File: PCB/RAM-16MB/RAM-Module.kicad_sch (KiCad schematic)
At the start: 0 parts

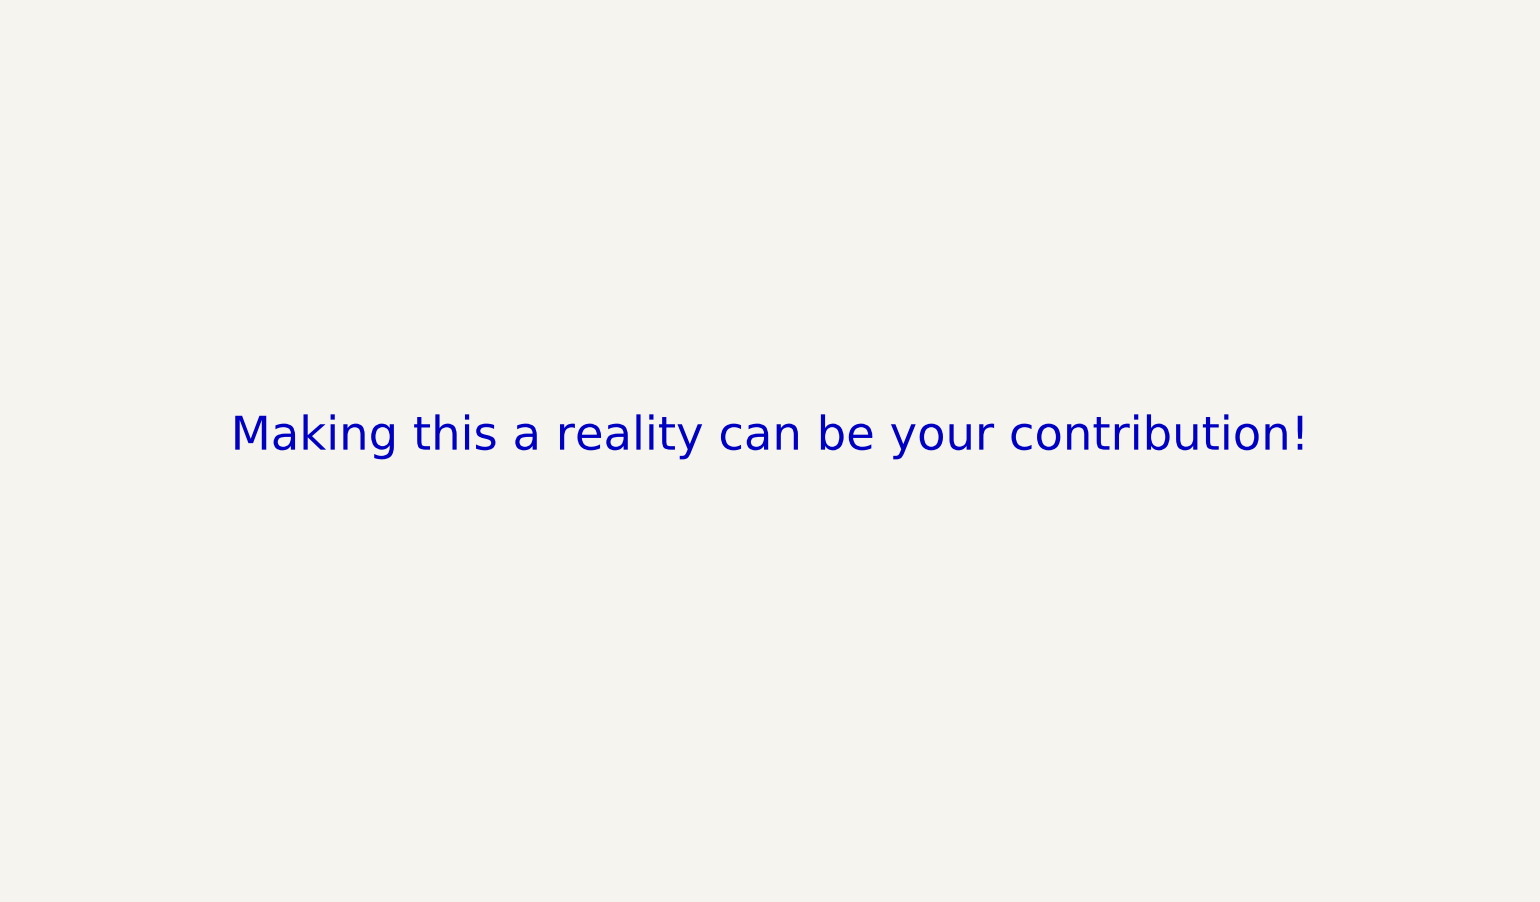
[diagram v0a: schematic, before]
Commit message: Add files via upload
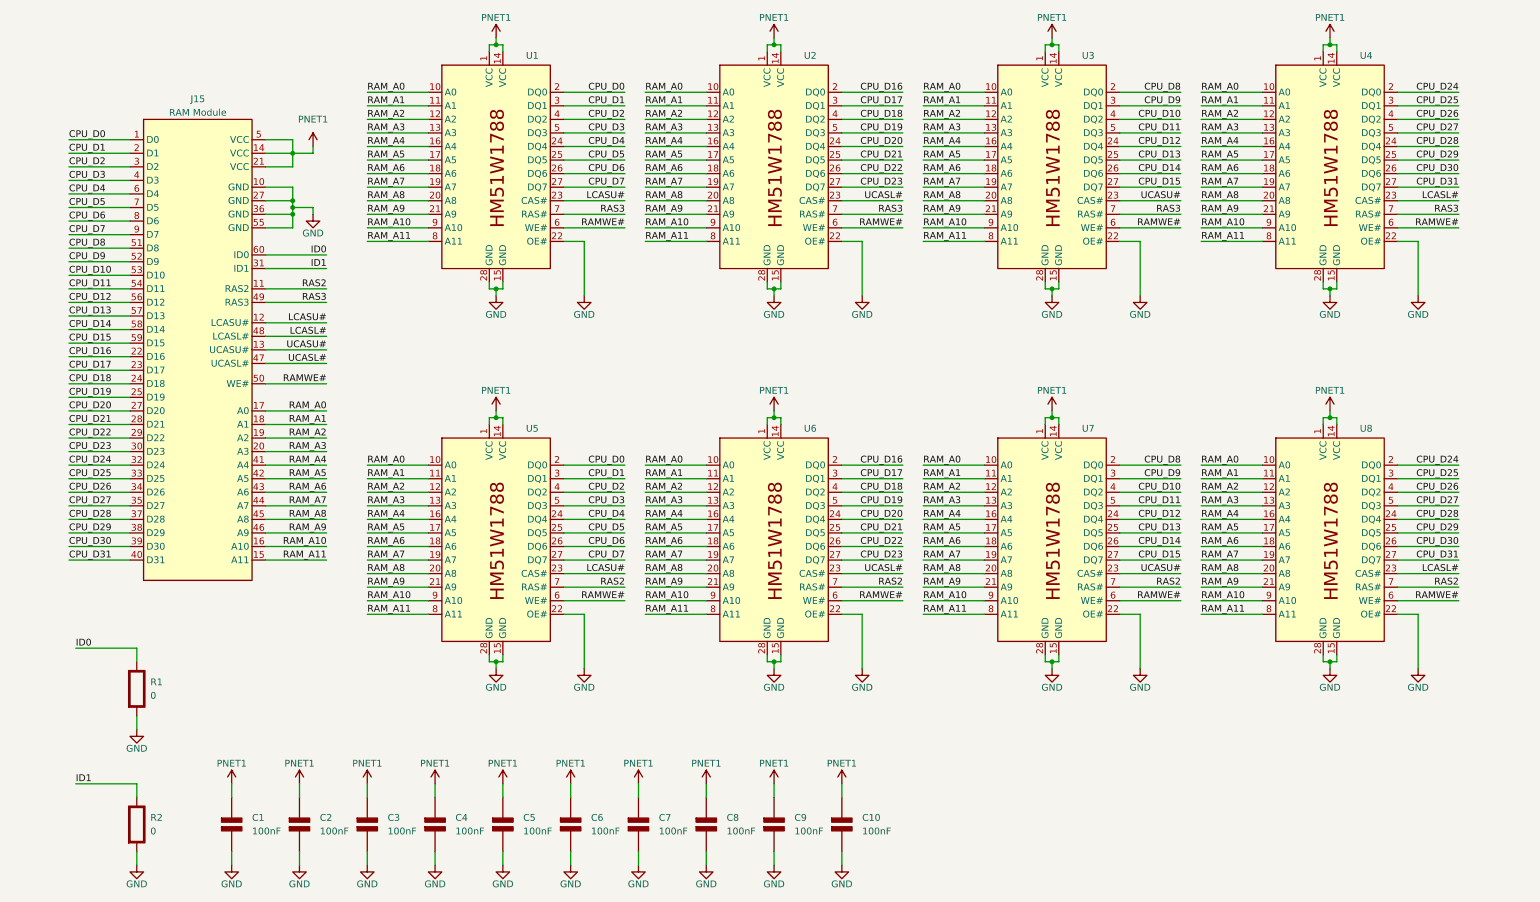
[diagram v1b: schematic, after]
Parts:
- added C1, C10, C2, C3, C4, C5, C6, C7, C8, C9: 100nF, symbol PCM_Elektuur:C
- added J15: RAM Module, symbol PC110:RAM_MOD
- added R1, R2: 0, symbol PCM_Elektuur:R
- added U1, U2, U3, U4, U5, U6, U7, U8: ~, symbol RAM-Module:HM51W1788
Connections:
- new net CPU_D0: J15.1 (D0), U1.2 (DQ0), U5.2 (DQ0)
- new net CPU_D1: J15.2 (D1), U1.3 (DQ1), U5.3 (DQ1)
- new net CPU_D10: J15.53 (D10), U3.4 (DQ2), U7.4 (DQ2)
- new net CPU_D11: J15.54 (D11), U3.5 (DQ3), U7.5 (DQ3)
- new net CPU_D12: J15.56 (D12), U3.24 (DQ4), U7.24 (DQ4)
- new net CPU_D13: J15.57 (D13), U3.25 (DQ5), U7.25 (DQ5)
- new net CPU_D14: J15.58 (D14), U3.26 (DQ6), U7.26 (DQ6)
- new net CPU_D15: J15.59 (D15), U3.27 (DQ7), U7.27 (DQ7)
- new net CPU_D16: J15.22 (D16), U2.2 (DQ0), U6.2 (DQ0)
- new net CPU_D17: J15.23 (D17), U2.3 (DQ1), U6.3 (DQ1)
- new net CPU_D18: J15.24 (D18), U2.4 (DQ2), U6.4 (DQ2)
- new net CPU_D19: J15.25 (D19), U2.5 (DQ3), U6.5 (DQ3)
- new net CPU_D2: J15.3 (D2), U1.4 (DQ2), U5.4 (DQ2)
- new net CPU_D20: J15.27 (GND), U2.24 (DQ4), U6.24 (DQ4)
- new net CPU_D21: J15.28 (D21), U2.25 (DQ5), U6.25 (DQ5)
- new net CPU_D22: J15.29 (D22), U2.26 (DQ6), U6.26 (DQ6)
- new net CPU_D23: J15.30 (D23), U2.27 (DQ7), U6.27 (DQ7)
- new net CPU_D24: J15.32 (D24), U4.2 (DQ0), U8.2 (DQ0)
- new net CPU_D25: J15.33 (D25), U4.3 (DQ1), U8.3 (DQ1)
- new net CPU_D26: J15.34 (D26), U4.4 (DQ2), U8.4 (DQ2)
- new net CPU_D27: J15.35 (D27), U4.5 (DQ3), U8.5 (DQ3)
- new net CPU_D28: J15.37 (D28), U4.24 (DQ4), U8.24 (DQ4)
- new net CPU_D29: J15.38 (D29), U4.25 (DQ5), U8.25 (DQ5)
- new net CPU_D3: J15.4 (D3), U1.5 (DQ3), U5.5 (DQ3)
- new net CPU_D30: J15.39 (D30), U4.26 (DQ6), U8.26 (DQ6)
- new net CPU_D31: J15.40 (D31), U4.27 (DQ7), U8.27 (DQ7)
- new net CPU_D4: J15.6 (D4), U1.24 (DQ4), U5.24 (DQ4)
- new net CPU_D5: J15.7 (D5), U1.25 (DQ5), U5.25 (DQ5)
- new net CPU_D6: J15.8 (D6), U1.26 (DQ6), U5.26 (DQ6)
- new net CPU_D7: J15.9 (D7), U1.27 (DQ7), U5.27 (DQ7)
- new net CPU_D8: J15.51 (D8), U3.2 (DQ0), U7.2 (DQ0)
- new net CPU_D9: J15.52 (D9), U3.3 (DQ1), U7.3 (DQ1)
- new net GND: C1.2 (-), C10.2 (-), C2.2 (-), C3.2 (-), C4.2 (-), C5.2 (-), C6.2 (-), C7.2 (-), C8.2 (-), C9.2 (-), J15.10 (GND), J15.27 (GND), J15.36 (GND), J15.55 (GND), R1.2 (-), R2.2 (-), U1.15 (GND), U1.22 (OE#), U1.28 (GND), U2.15 (GND), U2.22 (OE#), U2.28 (GND), U3.15 (GND), U3.22 (OE#), U3.28 (GND), U4.15 (GND), U4.22 (OE#), U4.28 (GND), U5.15 (GND), U5.22 (OE#), U5.28 (GND), U6.15 (GND), U6.22 (OE#), U6.28 (GND), U7.15 (GND), U7.22 (OE#), U7.28 (GND), U8.15 (GND), U8.22 (OE#), U8.28 (GND)
- new net ID0: J15.60 (ID0), R1.1 (+)
- new net ID1: J15.31 (ID1), R2.1 (+)
- new net LCASL#: J15.48 (LCASL#), U4.23 (CAS#), U8.23 (CAS#)
- new net LCASU#: J15.12 (LCASU#), U1.23 (CAS#), U5.23 (CAS#)
- new net PNET1: C1.1 (+), C10.1 (+), C2.1 (+), C3.1 (+), C4.1 (+), C5.1 (+), C6.1 (+), C7.1 (+), C8.1 (+), C9.1 (+), J15.14 (VCC), J15.21 (VCC), J15.5 (VCC), U1.1 (VCC), U1.14 (VCC), U2.1 (VCC), U2.14 (VCC), U3.1 (VCC), U3.14 (VCC), U4.1 (VCC), U4.14 (VCC), U5.1 (VCC), U5.14 (VCC), U6.1 (VCC), U6.14 (VCC), U7.1 (VCC), U7.14 (VCC), U8.1 (VCC), U8.14 (VCC)
- new net RAMWE#: J15.50 (WE#), U1.6 (WE#), U2.6 (WE#), U3.6 (WE#), U4.6 (WE#), U5.6 (WE#), U6.6 (WE#), U7.6 (WE#), U8.6 (WE#)
- new net RAM_A0: J15.17 (A0), U1.10 (A0), U2.10 (A0), U3.10 (A0), U4.10 (A0), U5.10 (A0), U6.10 (A0), U7.10 (A0), U8.10 (A0)
- new net RAM_A1: J15.18 (A1), U1.11 (A1), U2.11 (A1), U3.11 (A1), U4.11 (A1), U5.11 (A1), U6.11 (A1), U7.11 (A1), U8.11 (A1)
- new net RAM_A10: J15.16 (A10), U1.9 (A10), U2.9 (A10), U3.9 (A10), U4.9 (A10), U5.9 (A10), U6.9 (A10), U7.9 (A10), U8.9 (A10)
- new net RAM_A11: J15.15 (A11), U1.8 (A11), U2.8 (A11), U3.8 (A11), U4.8 (A11), U5.8 (A11), U6.8 (A11), U7.8 (A11), U8.8 (A11)
- new net RAM_A2: J15.19 (A2), U1.12 (A2), U2.12 (A2), U3.12 (A2), U4.12 (A2), U5.12 (A2), U6.12 (A2), U7.12 (A2), U8.12 (A2)
- new net RAM_A3: J15.20 (A3), U1.13 (A3), U2.13 (A3), U3.13 (A3), U4.13 (A3), U5.13 (A3), U6.13 (A3), U7.13 (A3), U8.13 (A3)
- new net RAM_A4: J15.41 (A4), U1.16 (A4), U2.16 (A4), U3.16 (A4), U4.16 (A4), U5.16 (A4), U6.16 (A4), U7.16 (A4), U8.16 (A4)
- new net RAM_A5: J15.42 (A5), U1.17 (A5), U2.17 (A5), U3.17 (A5), U4.17 (A5), U5.17 (A5), U6.17 (A5), U7.17 (A5), U8.17 (A5)
- new net RAM_A6: J15.43 (A6), U1.18 (A6), U2.18 (A6), U3.18 (A6), U4.18 (A6), U5.18 (A6), U6.18 (A6), U7.18 (A6), U8.18 (A6)
- new net RAM_A7: J15.44 (A7), U1.19 (A7), U2.19 (A7), U3.19 (A7), U4.19 (A7), U5.19 (A7), U6.19 (A7), U7.19 (A7), U8.19 (A7)
- new net RAM_A8: J15.45 (A8), U1.20 (A8), U2.20 (A8), U3.20 (A8), U4.20 (A8), U5.20 (A8), U6.20 (A8), U7.20 (A8), U8.20 (A8)
- new net RAM_A9: J15.46 (A9), U1.21 (A9), U2.21 (A9), U3.21 (A9), U4.21 (A9), U5.21 (A9), U6.21 (A9), U7.21 (A9), U8.21 (A9)
- new net RAS2: J15.11 (RAS2), U5.7 (RAS#), U6.7 (RAS#), U7.7 (RAS#), U8.7 (RAS#)
- new net RAS3: J15.49 (RAS3), U1.7 (RAS#), U2.7 (RAS#), U3.7 (RAS#), U4.7 (RAS#)
- new net UCASL#: J15.47 (UCASL#), U2.23 (CAS#), U6.23 (CAS#)
- new net UCASU#: J15.13 (UCASU#), U3.23 (CAS#), U7.23 (CAS#)
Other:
- note removed: "Making this a reality can be your contribution!"
- company: (none) -> Recreated by: Ahmad Byagowi
- title: (none) -> 16MB RAM Module
